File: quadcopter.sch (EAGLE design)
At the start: 11 parts, among them J1 AVR_SPI_PRG_6NS, U1 ATMEGA128RFA1

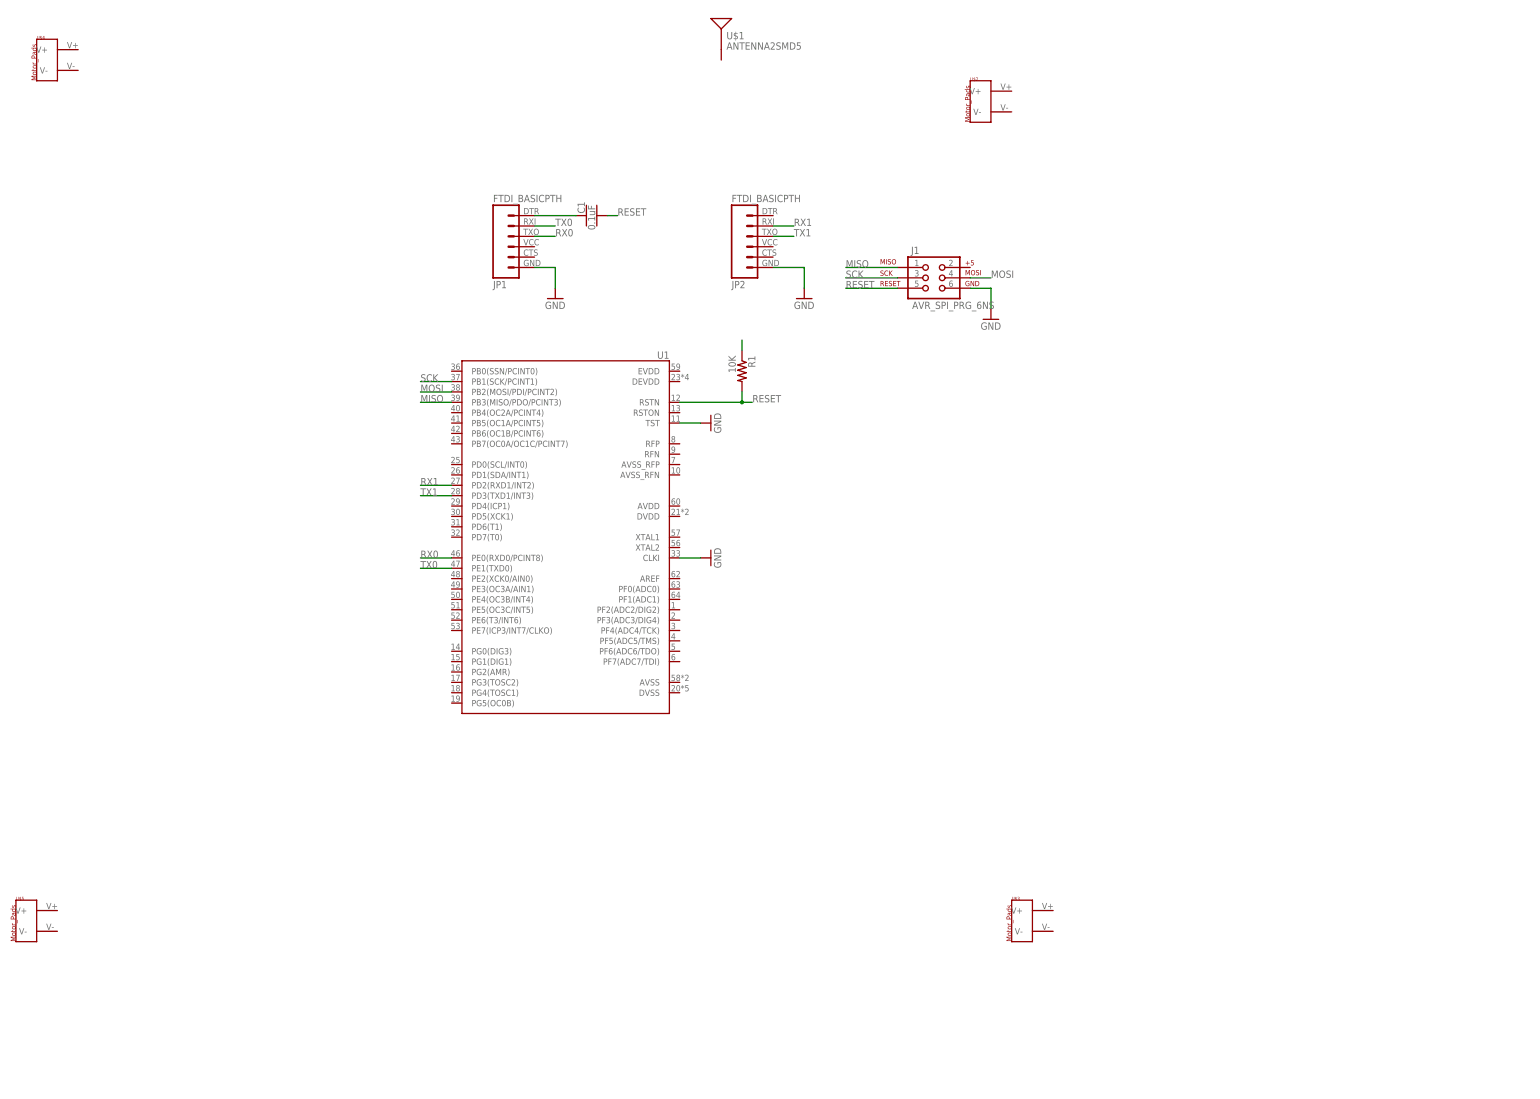
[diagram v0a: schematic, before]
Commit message: Sort of finished motor driver sch
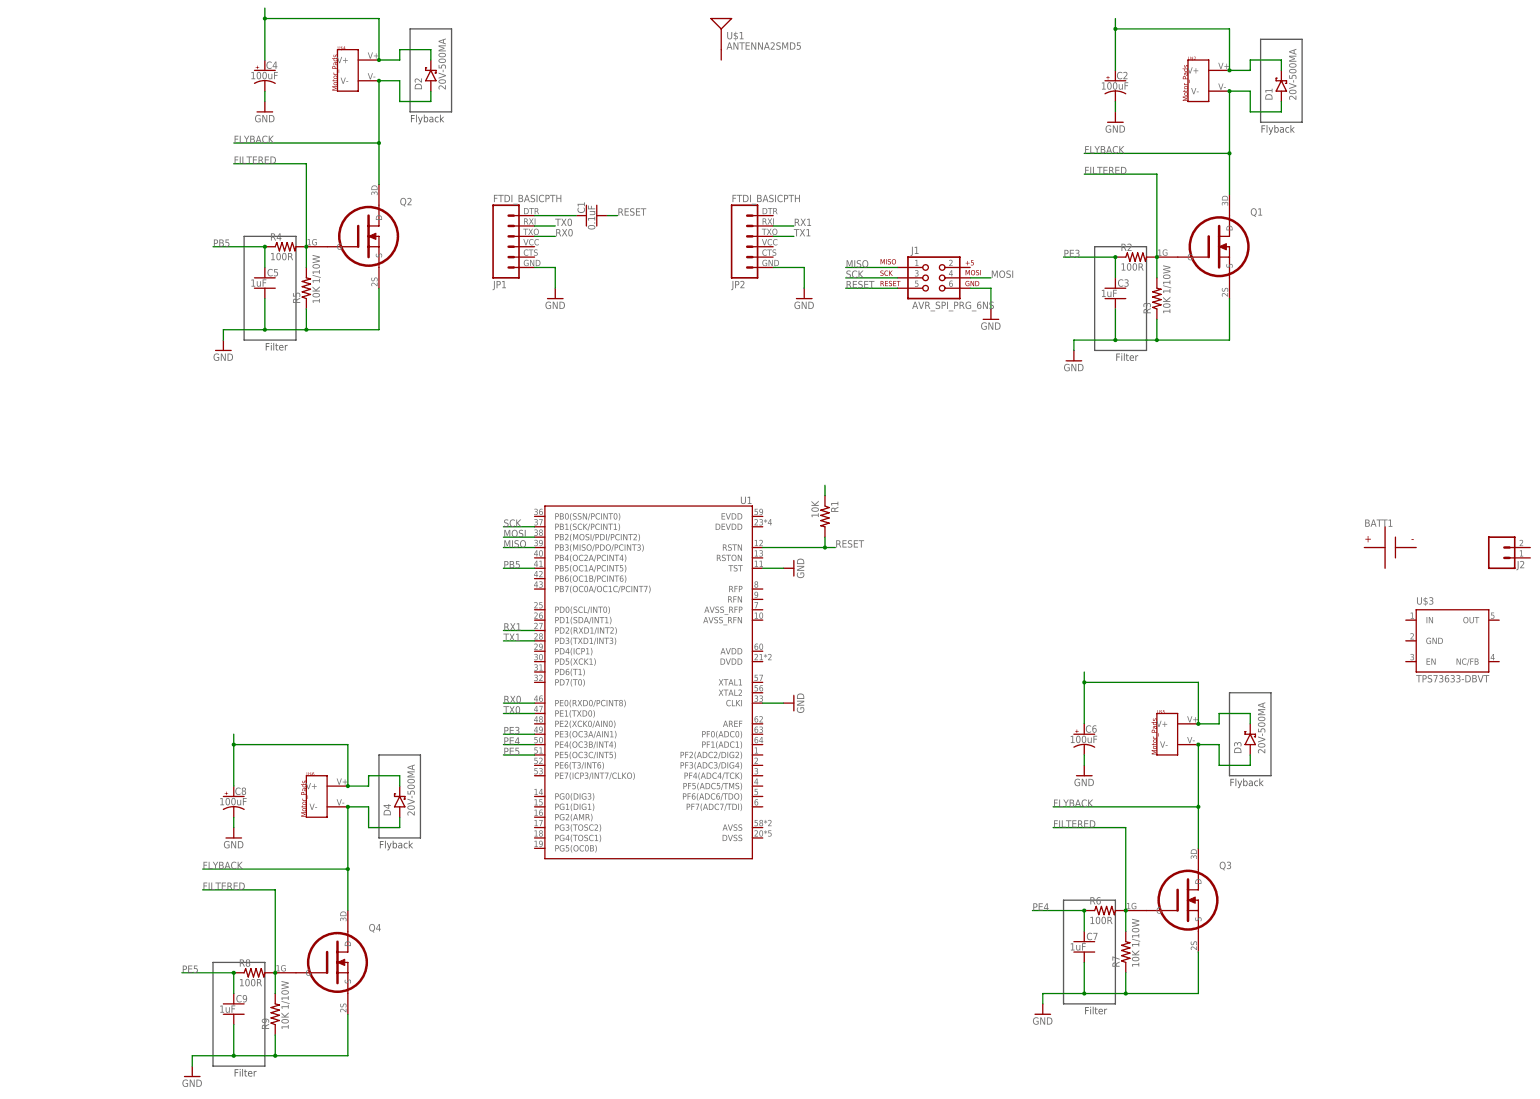
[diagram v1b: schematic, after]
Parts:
- added BATT1: BATTERY-HUBSAN-W/HOLDER, quadparts_prebuilt:BATTERY-HUBSAN-W/HOLDER
- added C2, C4, C6, C8: 100uF, quadparts_prebuilt:CAPACITOR-POL_SMD-7043-D_TANTALUM-220UF
- added C3, C5, C7, C9: 1uF, quadparts_prebuilt:CAPACITOR-NP_SMD-2012-0805_CERAMIC-1UF
- added D1, D2, D3, D4: 20V-500MA, quadparts_prebuilt:DIODE-SCHOTTKY_SMD-SOD123
- added J2: (no value), quadparts_connie:MALE_HEADER_2POS-2X1-0.1IN
- added Q1, Q2, Q3, Q4: (no value), quadparts_connie:N_MOSFET_SI2302CDS_T1_E3
- added R2, R4, R6, R8: 100R, quadparts_prebuilt:RESISTOR_SMD-2012-0805-100
- added R3, R5, R7, R9: 10K 1/10W, quadparts_prebuilt:RESISTOR_SMD-2012-0805-100
- added U$6: MOTOR_PADS, quadparts_prebuilt:MOTOR_PADS
- U$3: value MOTOR_PADS -> TPS73633-DBVT; device quadparts_prebuilt:MOTOR_PADS -> quadparts_prebuilt:TPS73633-DBVT
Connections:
- new net FILTERED: Q1.G, Q2.G, Q3.G, Q4.G, R2.2, R3.2, R4.2, R5.2, R6.2, R7.2, R8.2, R9.2
- new net FLYBACK: D1.A, D2.A, D3.A, D4.A, Q1.D, Q2.D, Q3.D, Q4.D, U$2.V-, U$4.V-, U$5.V-, U$6.V-
- new net N$10: C2.+, D1.C, U$2.V+
- new net N$13: C4.+, D2.C, U$4.V+
- new net N$14: C6.+, D3.C, U$5.V+
- new net N$15: C8.+, D4.C, U$6.V+
- new net N$16: U1.PB5(OC1A/PCINT5)
- new net PB5: C3.1, C5.1, C7.1, C9.1, R2.1, R4.1, R6.1, R8.1
- new net PE3: U1.PE3(OC3A/AIN1)
- new net PE4: U1.PE4(OC3B/INT4)
- new net PE5: U1.PE5(OC3C/INT5)
- net GND: now also C2.-, C3.2, C4.-, C5.2, C6.-, C7.2, C8.-, C9.2, Q1.S, Q2.S, Q3.S, Q4.S, R3.1, R5.1, R7.1, R9.1
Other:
- note added: "Filter"
- note added: "Flyback"
- moved on the sheet: R1, U$2, U$4, U$5, U1
